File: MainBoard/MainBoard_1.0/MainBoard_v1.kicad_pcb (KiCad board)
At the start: 2 copper layers, 120 x 80 mm, 165 parts, among them J1 ILG, J10 SH, J11 SH, J12 SH, J13 FFC, J14 SH, J2 SH, J3 STDC14, J4 PA, J5 Micro_SD_Card_Det_Hirose_DM3AT, J6 SH, J7 ENC, J8 ENC, J9 PA, Q1 AON7400B, Q10 IRLML6344, Q2 AON7400B, Q3 AON7400B, Q4 AON7400B, Q5 AON7400B, Q6 AON7400B, Q7 2N7002K, Q8 AON7400B, Q9 AON7400B, SW1 SKRPACE010, SW2 SSSS213202, SW3 FR01SC16P-S, SW4 SKRHAAE010, U1 SI7469DP-T1-GE3, U10 DRV8701E, U11 MMC5983MA, U2 LT1963A-TSSOP, U3 TPS62143, U4 ECS-2520S33, U5 INA260, U6 DRV8701E, U7 ICM20648, U8 STM32F469VG, U9 INA260

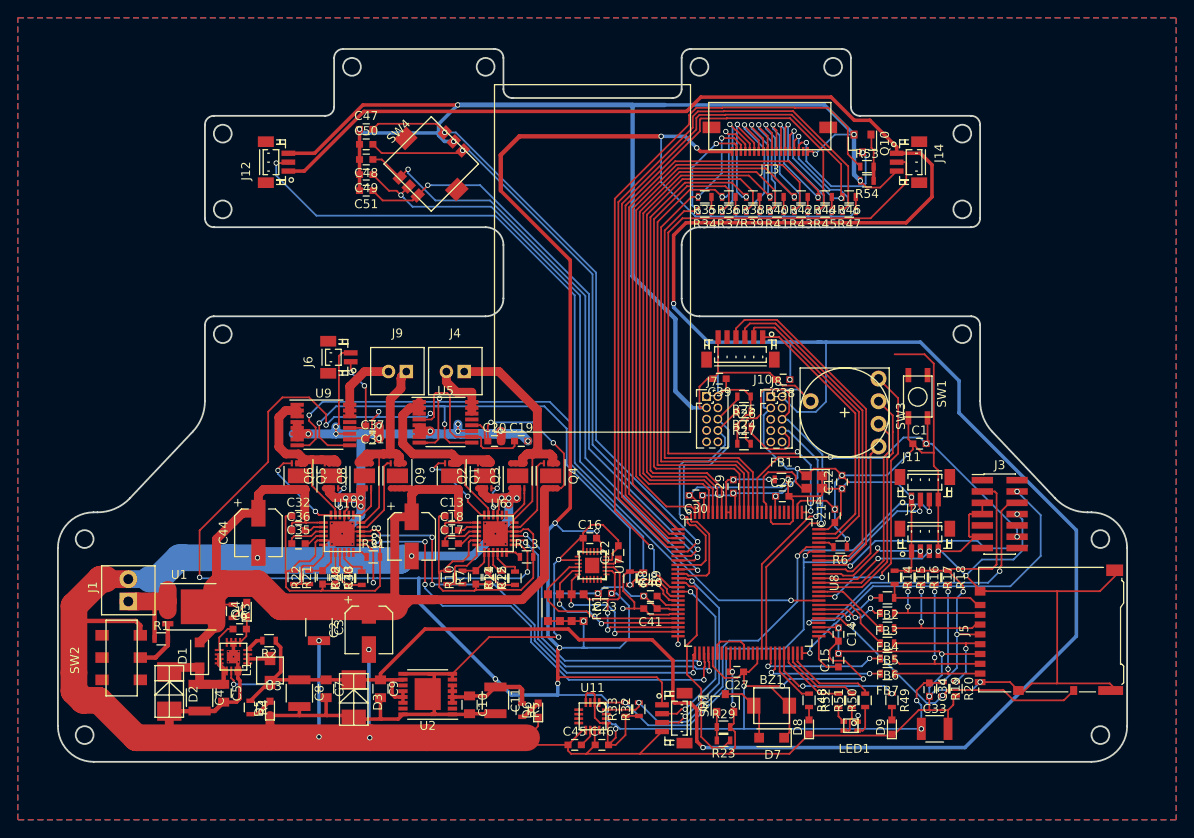
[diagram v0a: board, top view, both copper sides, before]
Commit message: fixed main_board
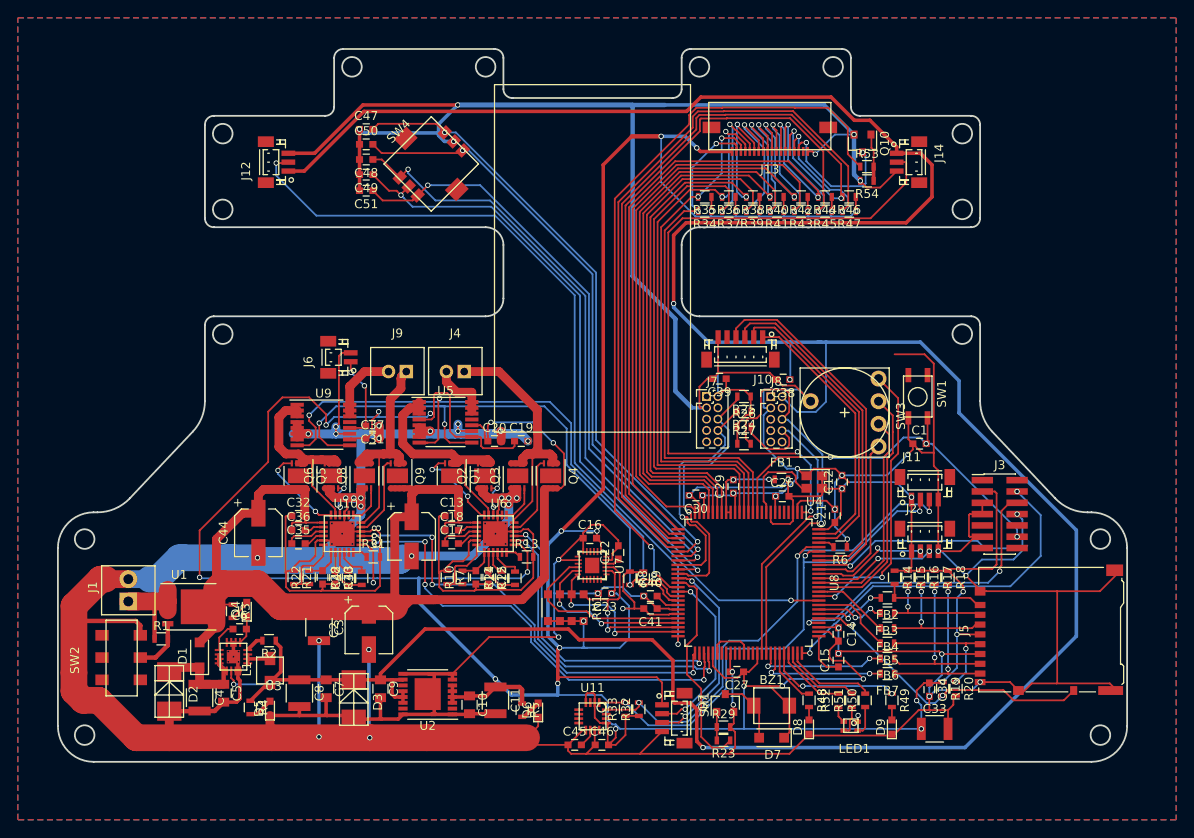
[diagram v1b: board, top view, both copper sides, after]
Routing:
- net +3V3: track 561.0 -> 546.1 mm
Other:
- outline, holes or cut-outs redrawn
